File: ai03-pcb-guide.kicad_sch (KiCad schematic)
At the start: 24 parts, among them U1 MOUDLE-SEEEDUINO-XIAO

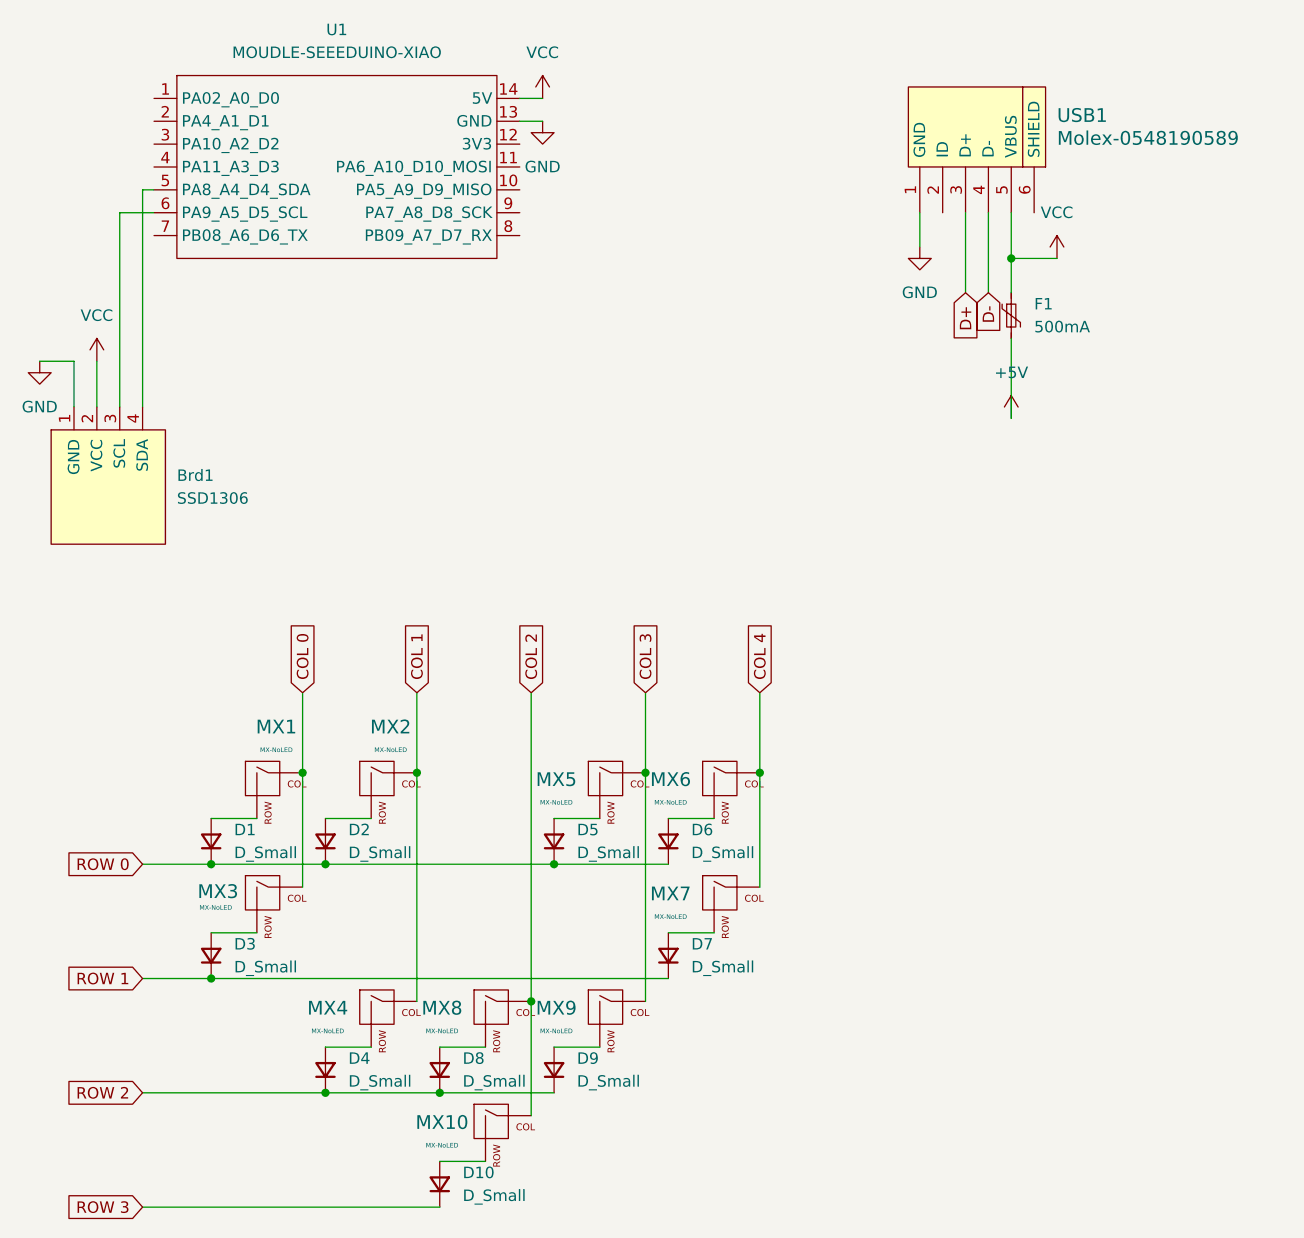
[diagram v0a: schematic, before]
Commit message: second commit of the day!
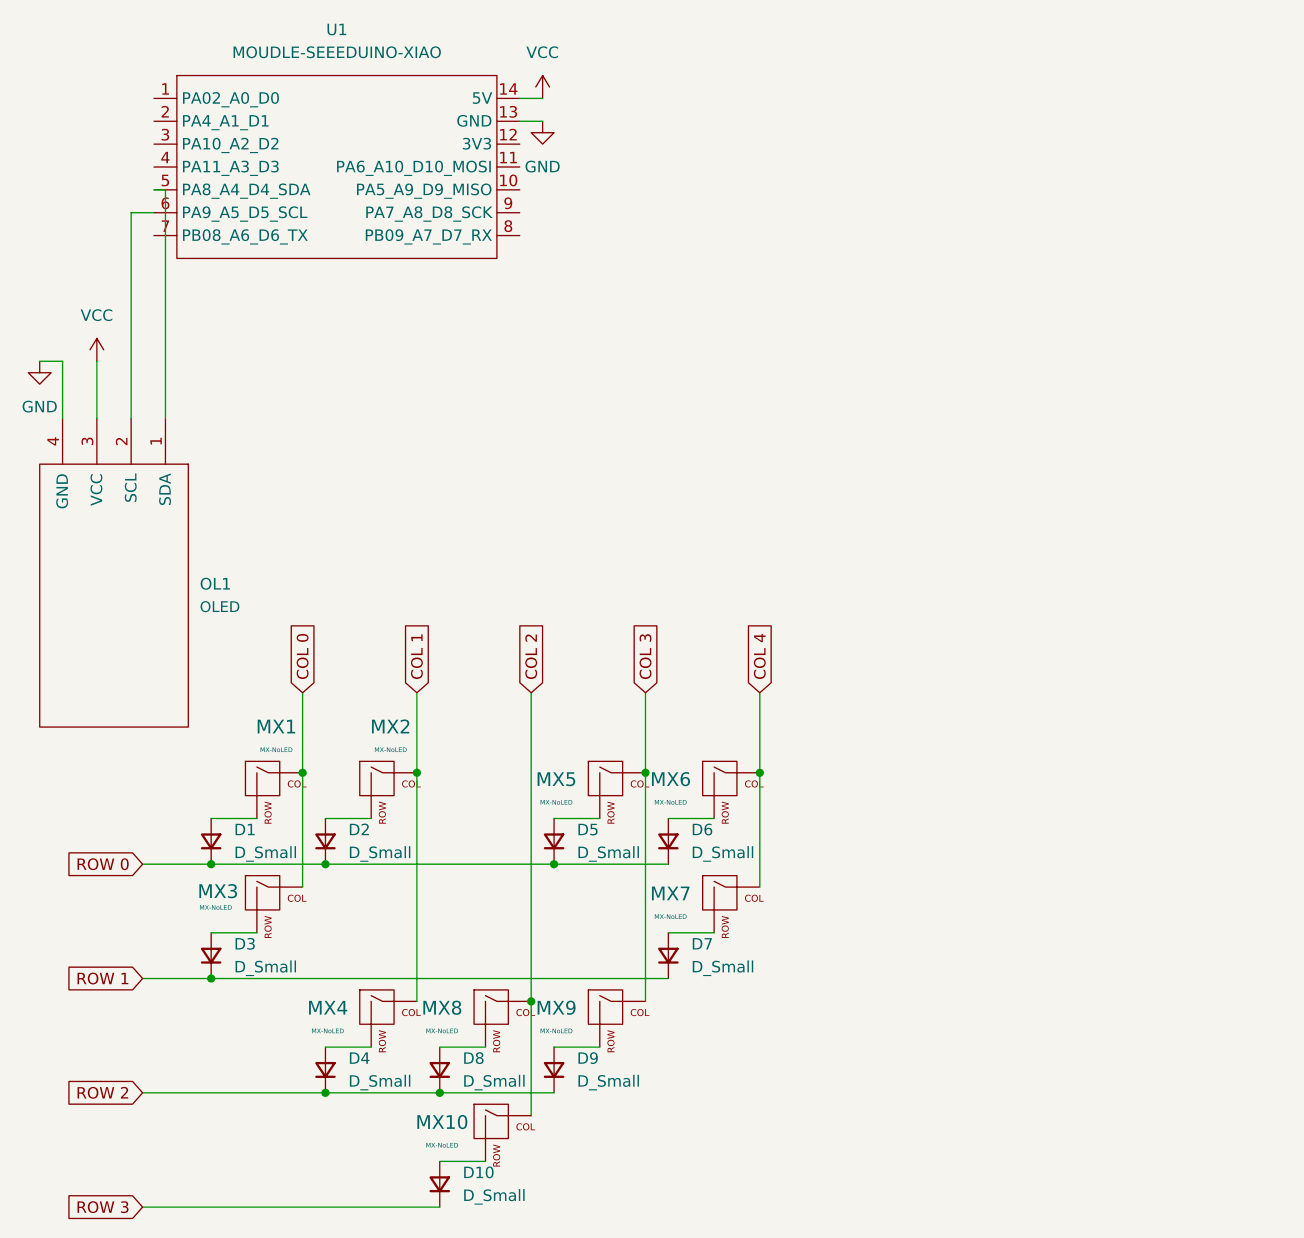
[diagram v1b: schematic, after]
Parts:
- removed Brd1: SSD1306, SSD1306:128x64OLED, symbol SSD1306-128x64_OLED:SSD1306
- removed F1: 500mA, Fuse:Fuse_1206_3216Metric, symbol Device:Polyfuse_Small
- removed USB1: Molex-0548190589, random-keyboard-parts:Molex-0548190589, symbol random-keyboard-parts:Molex-0548190589
- added OL1: OLED, kbd:OLED, symbol kbd:OLED
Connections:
- net GND: now also OL1.4 (GND)
- net VCC: now also OL1.3 (VCC)
- net at U1.5 (PA8_A4_D4_SDA): now also OL1.1 (SDA)
- net at U1.6 (PA9_A5_D5_SCL): now also OL1.2 (SCL)

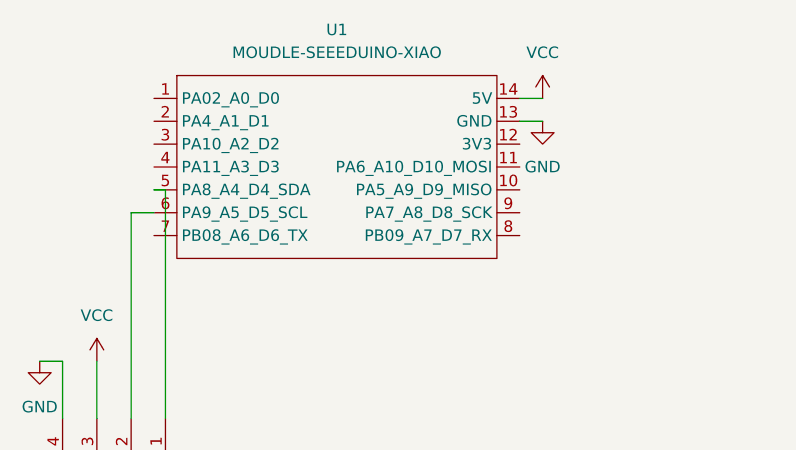
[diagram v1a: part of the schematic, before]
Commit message: yay
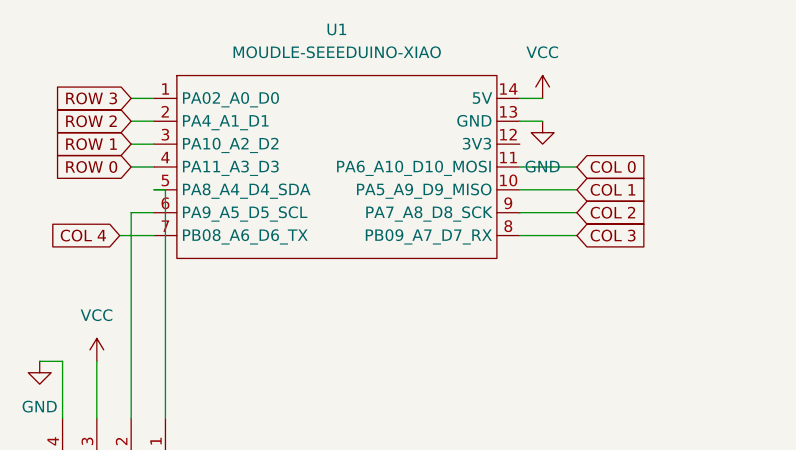
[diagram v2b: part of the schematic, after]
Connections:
- net COL 0: now also U1.11 (PA6_A10_D10_MOSI)
- net COL 1: now also U1.10 (PA5_A9_D9_MISO)
- net COL 2: now also U1.9 (PA7_A8_D8_SCK)
- net COL 3: now also U1.8 (PB09_A7_D7_RX)
- net COL 4: now also U1.7 (PB08_A6_D6_TX)
- net ROW 0: now also U1.4 (PA11_A3_D3)
- net ROW 1: now also U1.3 (PA10_A2_D2)
- net ROW 2: now also U1.2 (PA4_A1_D1)
- net ROW 3: now also U1.1 (PA02_A0_D0)

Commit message: a commit
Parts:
- MX1, MX10, MX2, MX3, MX4, MX5, MX6, MX7, MX8, MX9: footprint MX_Alps_Hybrid:MX-1U-NoLED -> Button_Switch_Keyboard:SW_Cherry_MX_1.00u_PCB
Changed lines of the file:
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@@
 			)
 		)
-		(property "Footprint" "MX_Alps_Hybrid:MX-1U-NoLED"
+		(property "Footprint" "Button_Switch_Keyboard:SW_Cherry_MX_1.00u_PCB"
 			(at 71.755 116.205 0)
 			(effects
@@
 			)
 		)
-		(property "Footprint" "MX_Alps_Hybrid:MX-1U-NoLED"
+		(property "Footprint" "Button_Switch_Keyboard:SW_Cherry_MX_1.00u_PCB"
 			(at 84.455 116.205 0)
 			(effects
@@
 			)
 		)
-		(property "Footprint" "MX_Alps_Hybrid:MX-1U-NoLED"
+		(property "Footprint" "Button_Switch_Keyboard:SW_Cherry_MX_1.00u_PCB"
 			(at 33.655 128.905 0)
 			(effects
@@
 			)
 		)
-		(property "Footprint" "MX_Alps_Hybrid:MX-1U-NoLED"
+		(property "Footprint" "Button_Switch_Keyboard:SW_Cherry_MX_1.00u_PCB"
 			(at 84.455 128.905 0)
 			(effects
@@
 			)
 		)
-		(property "Footprint" "MX_Alps_Hybrid:MX-1U-NoLED"
+		(property "Footprint" "Button_Switch_Keyboard:SW_Cherry_MX_1.00u_PCB"
 			(at 46.355 116.205 0)
 			(effects
@@
 			)
 		)
-		(property "Footprint" "MX_Alps_Hybrid:MX-1U-NoLED"
+		(property "Footprint" "Button_Switch_Keyboard:SW_Cherry_MX_1.00u_PCB"
 			(at 59.055 154.305 0)
 			(effects
@@
 			)
 		)
-		(property "Footprint" "MX_Alps_Hybrid:MX-1U-NoLED"
+		(property "Footprint" "Button_Switch_Keyboard:SW_Cherry_MX_1.00u_PCB"
 			(at 59.055 141.605 0)
 			(effects
@@
 			)
 		)
-		(property "Footprint" "MX_Alps_Hybrid:MX-1U-NoLED"
+		(property "Footprint" "Button_Switch_Keyboard:SW_Cherry_MX_1.00u_PCB"
 			(at 71.755 141.605 0)
 			(effects
@@
 			)
 		)
-		(property "Footprint" "MX_Alps_Hybrid:MX-1U-NoLED"
+		(property "Footprint" "Button_Switch_Keyboard:SW_Cherry_MX_1.00u_PCB"
 			(at 46.355 141.605 0)
 			(effects
@@
 			)
 		)
-		(property "Footprint" "MX_Alps_Hybrid:MX-1U-NoLED"
+		(property "Footprint" "Button_Switch_Keyboard:SW_Cherry_MX_1.00u_PCB"
 			(at 33.655 116.205 0)
 			(effects
